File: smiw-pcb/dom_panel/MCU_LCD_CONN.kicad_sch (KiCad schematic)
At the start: 1 part, among them J1 4-1734839-5

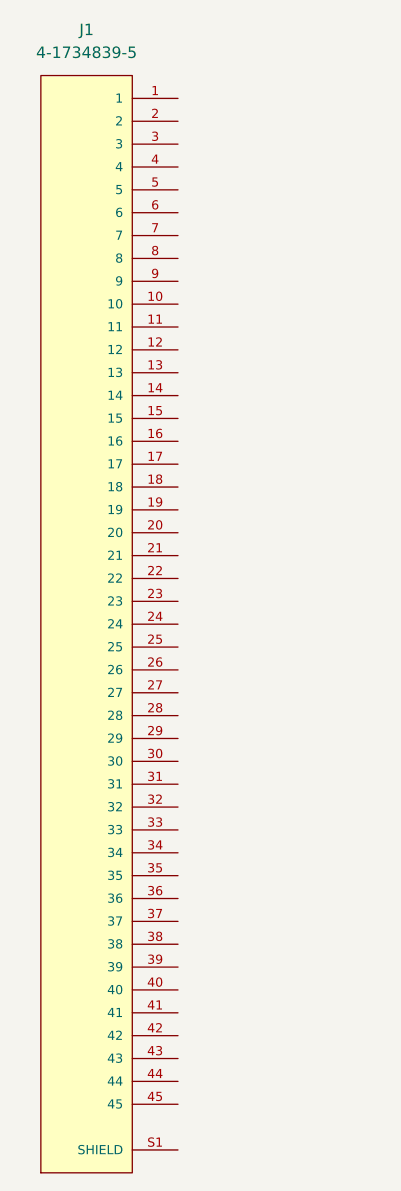
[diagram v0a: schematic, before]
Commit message: cos
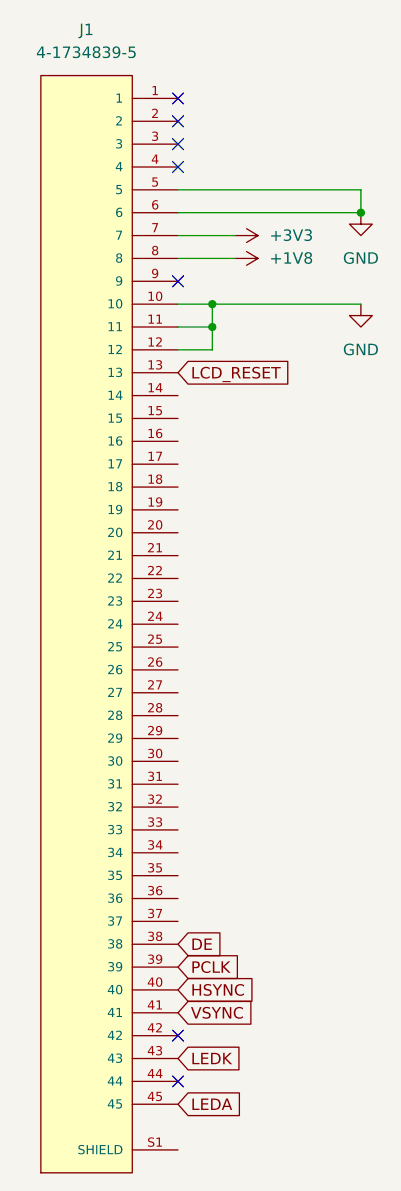
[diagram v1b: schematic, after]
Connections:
- net GND: now reaches J1.10
- net GND: now also J1.11, J1.12, J1.5, J1.6
- net LCD_RESET: now reaches J1.13
- net DE: now reaches J1.38
- net PCLK: now reaches J1.39
- net HSYNC: now reaches J1.40
- net VSYNC: now reaches J1.41
- net LEDK: now reaches J1.43
- net LEDA: now reaches J1.45
- net +3V3: now reaches J1.7
- net +1V8: now reaches J1.8
- no-connect marks 0 -> 7
